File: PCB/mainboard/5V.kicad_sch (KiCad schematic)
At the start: 12 parts, among them U1 TPS5430DDA

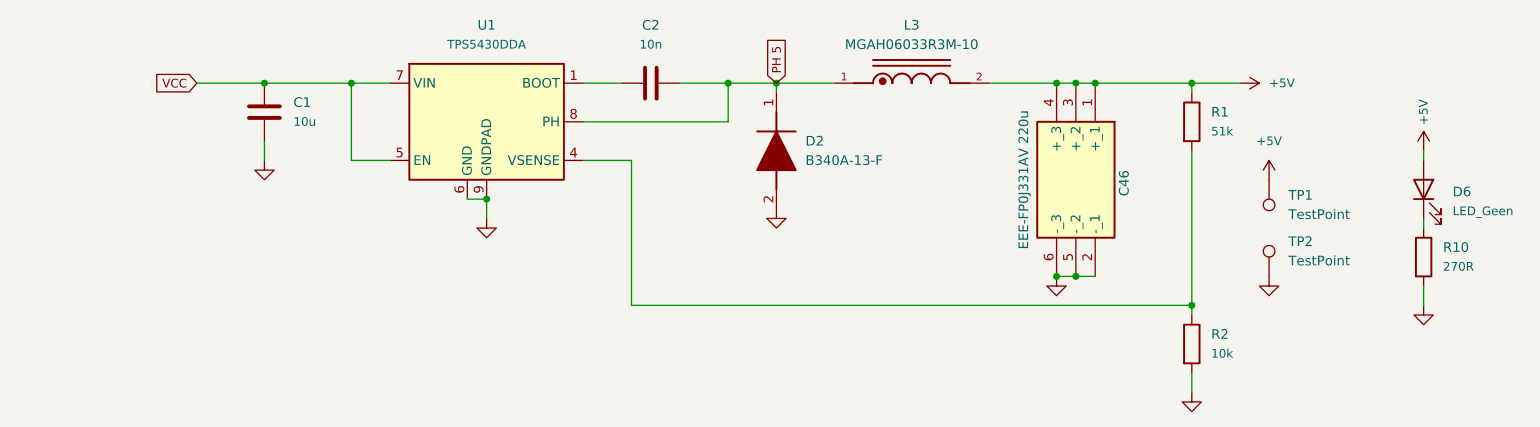
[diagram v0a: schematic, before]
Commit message: random upload
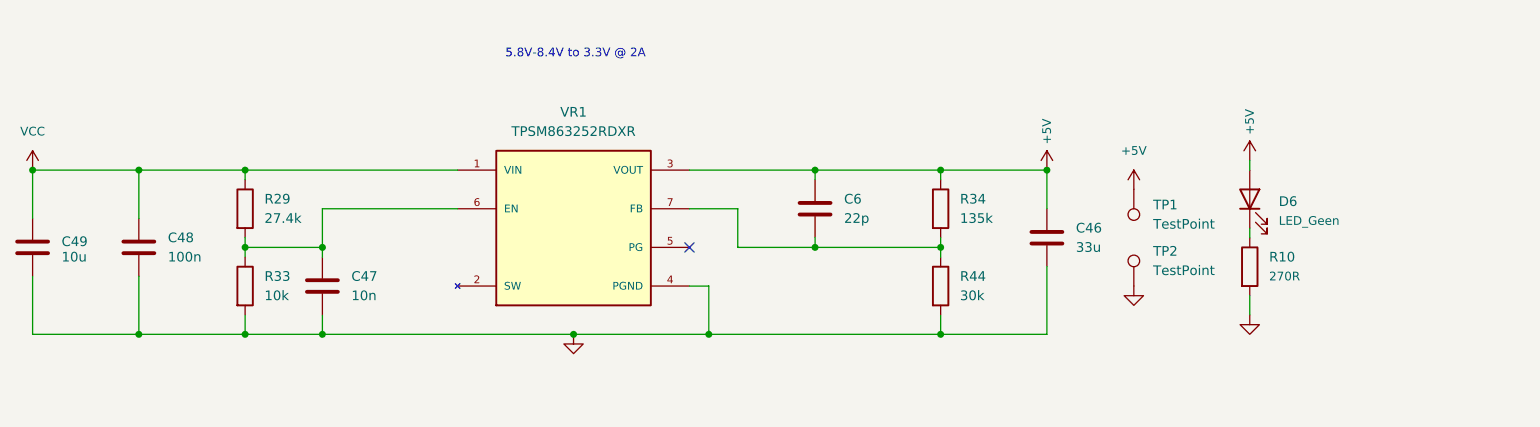
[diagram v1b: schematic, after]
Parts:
- removed C1: 10u, Capacitor_SMD:C_1206_3216Metric_Pad1.33x1.80mm_HandSolder, symbol Device:C
- removed C2: 10n, Capacitor_SMD:C_1206_3216Metric_Pad1.33x1.80mm_HandSolder, symbol Device:C
- removed C46: EEE-FP0J331AV 220u, lib:EEEFP0J331AV, symbol EEE-FP0J331AV:EEE-FP0J331AV
- removed D2: B340A-13-F, lib:DIOM5226X240N, symbol B340A-13-F:B340A-13-F
- removed L3: MGAH06033R3M-10, lib:IND_MGAH06033R3M-10, symbol MGAH06033R3M-10:MGAH06033R3M-10
- removed R1: 51k, Resistor_SMD:R_0402_1005Metric_Pad0.72x0.64mm_HandSolder, symbol Device:R
- removed R2: 10k, Resistor_SMD:R_0402_1005Metric_Pad0.72x0.64mm_HandSolder, symbol Device:R
- removed U1: TPS5430DDA, Package_SO:TI_SO-PowerPAD-8_ThermalVias, symbol Regulator_Switching:TPS5430DDA
- added C46: 33u, lib:C4532_Commercial, symbol Device:C
- added C47: 10n, Capacitor_SMD:C_0402_1005Metric_Pad0.74x0.62mm_HandSolder, symbol Device:C
- added C48: 100n, Capacitor_SMD:C_0402_1005Metric_Pad0.74x0.62mm_HandSolder, symbol Device:C
- added C49: 10u, Capacitor_SMD:C_0402_1005Metric_Pad0.74x0.62mm_HandSolder, symbol Device:C
- added C6: 22p, Capacitor_SMD:C_0402_1005Metric_Pad0.74x0.62mm_HandSolder, symbol Device:C
- added R29: 27.4k, Resistor_SMD:R_0402_1005Metric_Pad0.72x0.64mm_HandSolder, symbol Device:R
- added R33: 10k, Resistor_SMD:R_0402_1005Metric_Pad0.72x0.64mm_HandSolder, symbol Device:R
- added R34: 135k, Resistor_SMD:R_0402_1005Metric_Pad0.72x0.64mm_HandSolder, symbol Device:R
- added R44: 30k, Resistor_SMD:R_0402_1005Metric_Pad0.72x0.64mm_HandSolder, symbol Device:R
- added VR1: TPSM863252RDXR, lib:VREG_TPSM863252RDXR, symbol TPSM863252RDXR:TPSM863252RDXR
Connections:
- net +5V: now also C46.1, C6.1, R34.1, VR1.3 (VOUT)
- net GND: now also C46.2, C47.2, C48.2, C49.2, R33.2, R44.2, VR1.4 (PGND)
- net VCC: now also C48.1, C49.1, R29.1, VR1.1 (VIN)
- new net: C47.1, R29.2, R33.1, VR1.6 (EN)
- new net: C6.2, R34.2, R44.1, VR1.7 (FB)
- no-connect marks 0 -> 1
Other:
- note added: "5.8V-8.4V to 3.3V @ 2A"
- moved on the sheet: D6, R10, TP1, TP2
